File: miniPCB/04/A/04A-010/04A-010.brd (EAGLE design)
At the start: 29 parts

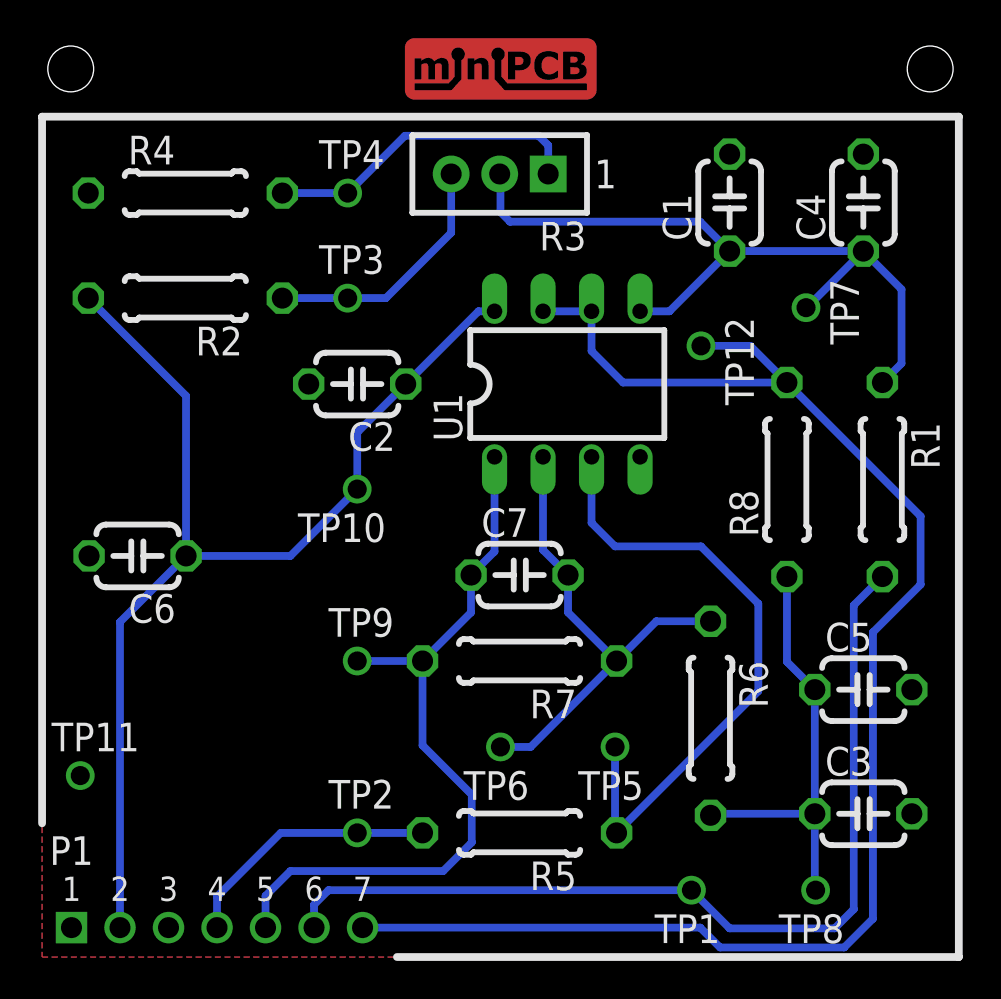
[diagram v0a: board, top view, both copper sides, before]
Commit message: NM.14JAN2023
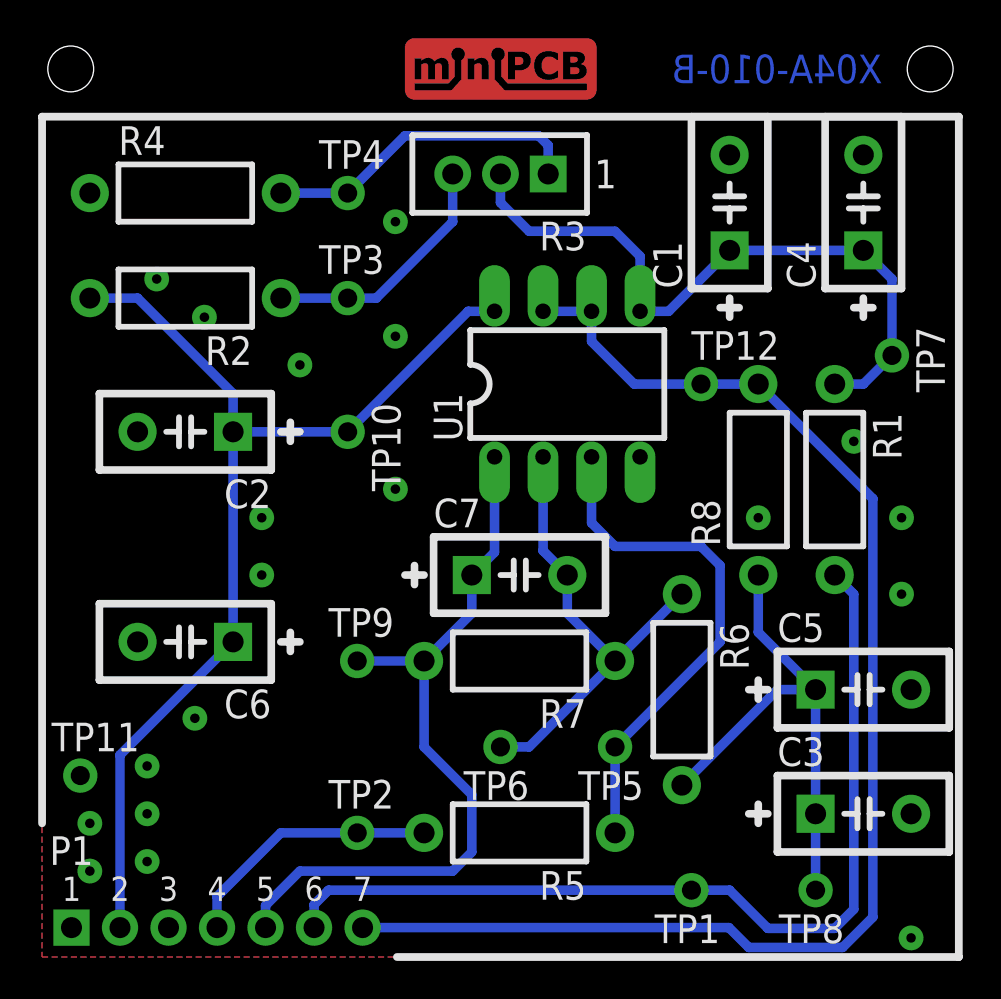
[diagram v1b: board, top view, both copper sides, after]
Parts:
- moved C2 9.34 mm to (8.50, 28.5)
- moved C6 5.15 mm to (8.50, 17.5)
- moved TP7 5.15 mm to (45.5, 32.5)
- moved TP10 3.04 mm to (17.0, 28.5), turned to 270 degrees
- moved R1 2.50 mm to (42.5, 26.0)
- moved R6 2.12 mm to (34.5, 15.0)
- moved TP12 2.00 mm to (35.5, 31.0)
- moved R8 1.50 mm to (38.5, 26.0)
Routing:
- net VREF: track 80.6 -> 72.0 mm
- net IN+: track 33.5 -> 27.4 mm
- net BIAS: track 40.2 -> 35.6 mm
- net VREF_FILTERED: track 22.5 -> 26.8 mm
- net V+: track 59.7 -> 56.3 mm
- net VFB: track 26.0 -> 25.1 mm
